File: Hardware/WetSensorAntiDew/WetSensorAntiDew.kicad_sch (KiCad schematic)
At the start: 22 parts, among them J1 Teensy Connector, J2 Connector to BME280, J3 1-4 to HeatedWetSensor | 5-7 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, J4 Teensy Connector, J5 Connector to power supply, J6 Connector to power supply, Q1 MOSFET N-CH, U1 AMS1117

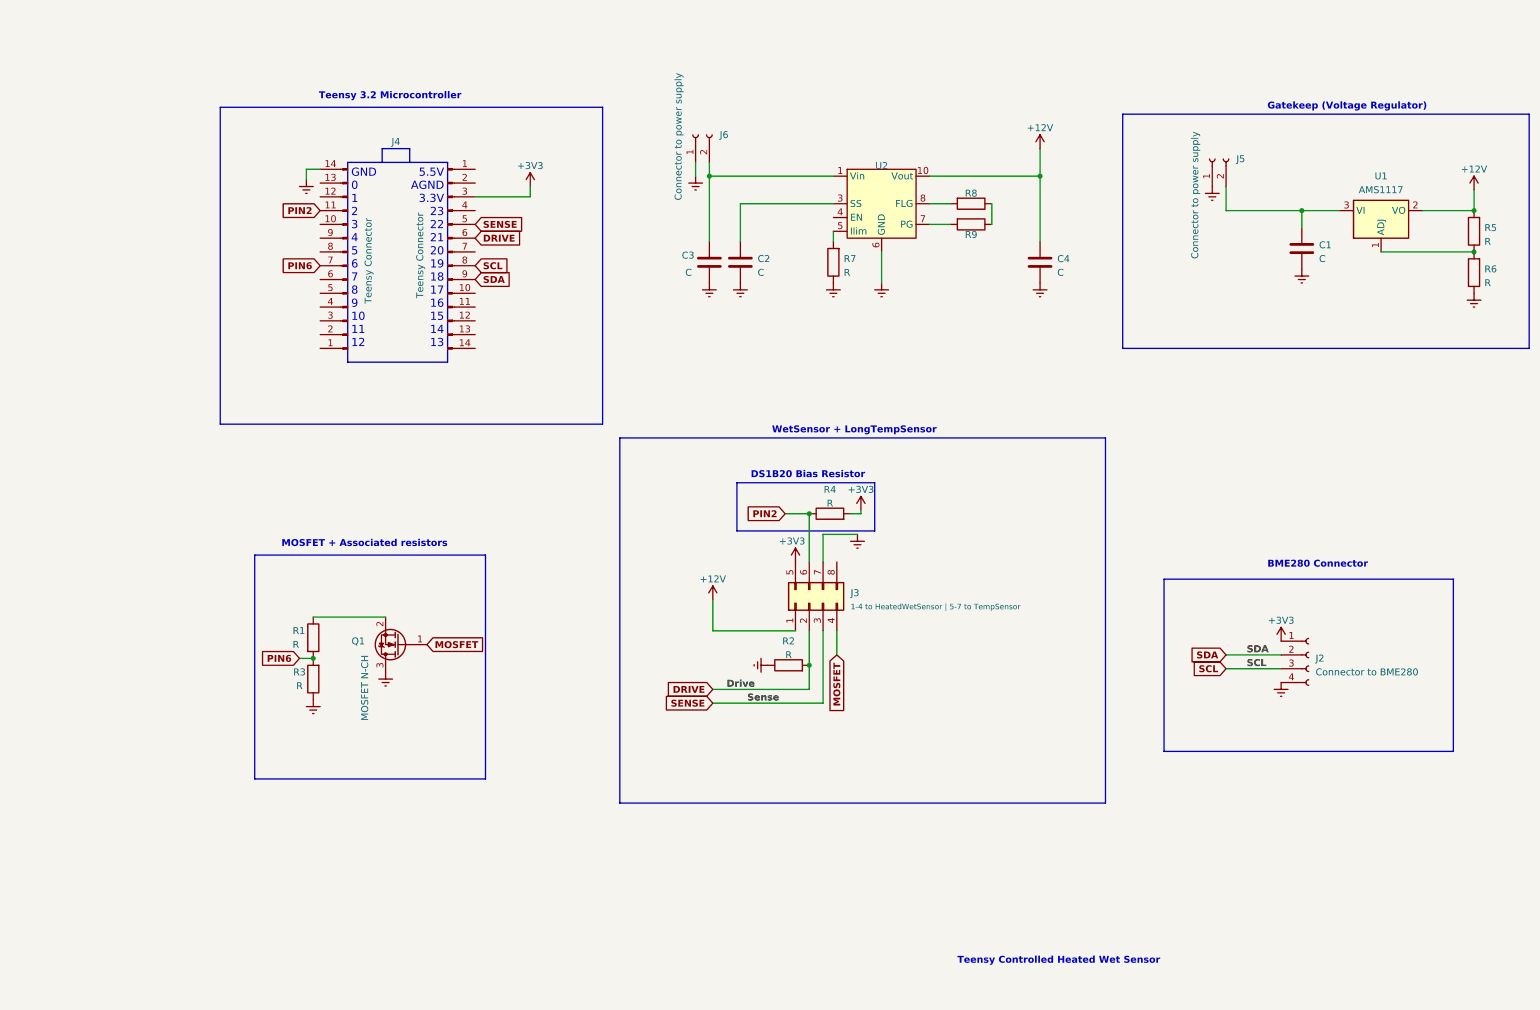
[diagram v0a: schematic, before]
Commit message: changes
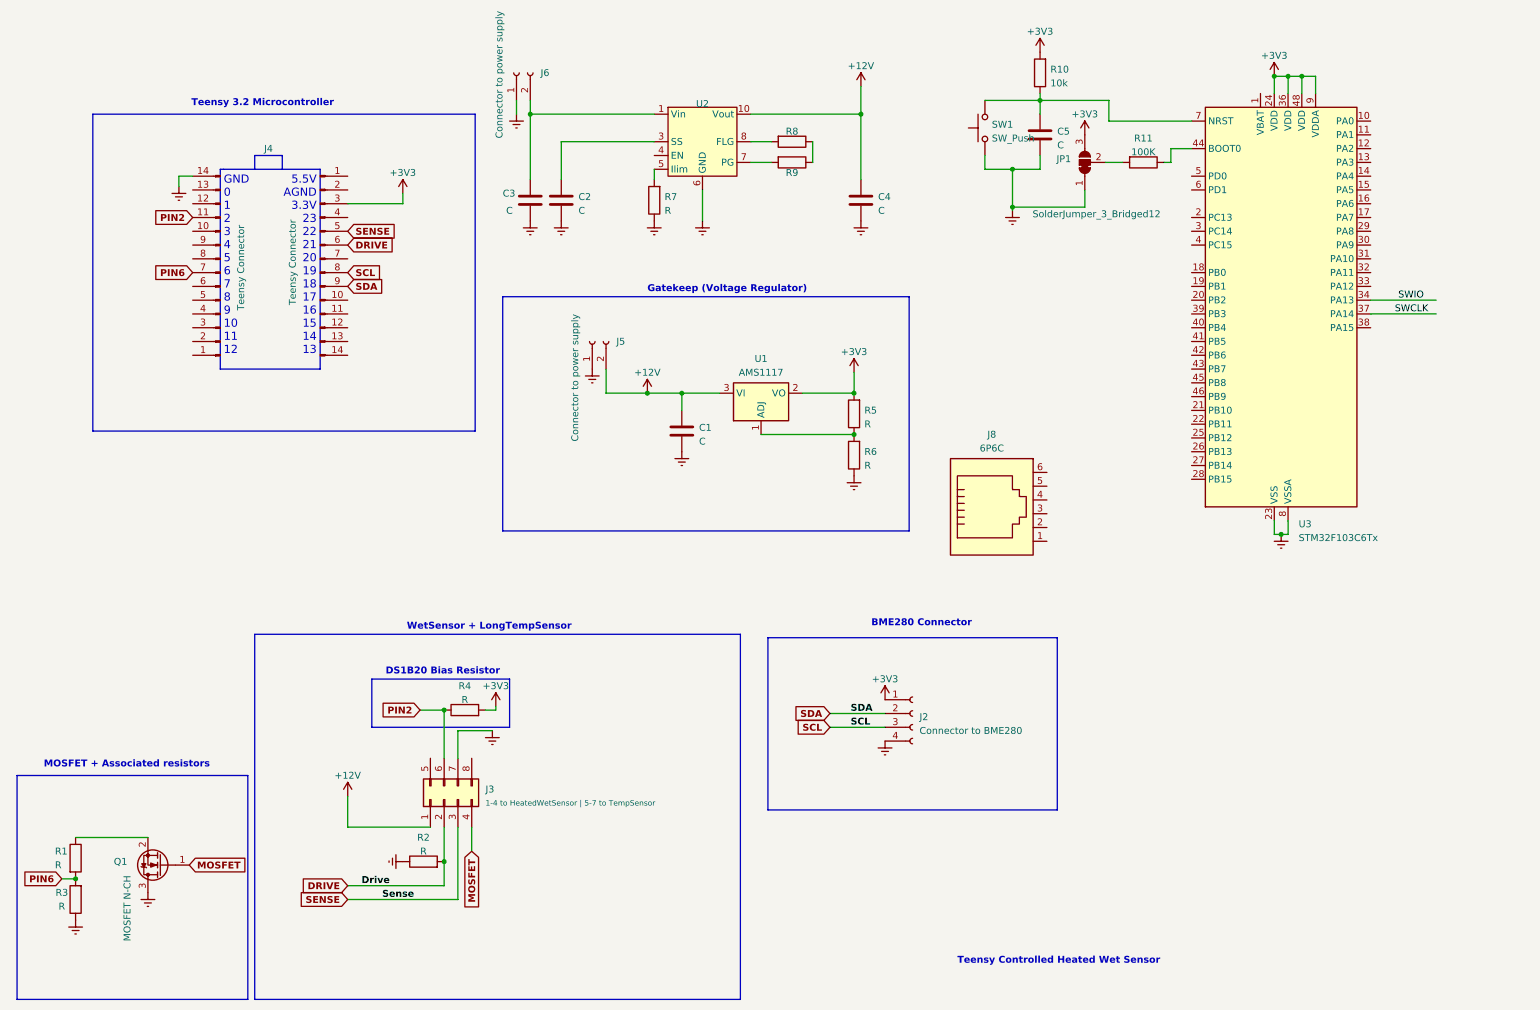
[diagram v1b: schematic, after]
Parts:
- added C5: C, Capacitor_SMD:C_0603_1608Metric_Pad1.08x0.95mm_HandSolder, symbol Device:C
- added J8: 6P6C, Connector_RJ:RJ12_Amphenol_54601, symbol Connector:6P6C
- added JP1: SolderJumper_3_Bridged12, Jumper:SolderJumper-3_P1.3mm_Bridged12_Pad1.0x1.5mm_NumberLabels, symbol Jumper:SolderJumper_3_Bridged12
- added R10: 10k, Resistor_SMD:R_0603_1608Metric_Pad0.98x0.95mm_HandSolder, symbol Device:R
- added R11: 100K, Resistor_SMD:R_0603_1608Metric_Pad0.98x0.95mm_HandSolder, symbol Device:R
- added SW1: SW_Push, symbol Switch:SW_Push
- added U3: STM32F103C6Tx, Package_QFP:LQFP-48_7x7mm_P0.5mm, symbol MCU_ST_STM32F1:STM32F103C6Tx
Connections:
- net +12V: now also C1.1, J5.2 (Pin_2), U1.3 (VI); no longer R5.2, U1.2 (VO)
- net +3V3: now also R5.2, U1.2 (VO), JP1.3 (B), R10.2, U3.24 (VDD), U3.36 (VDD), U3.48 (VDD), U3.9 (VDDA); no longer J3.5 (Pin_5)
- net Earth: now also C5.2, JP1.1 (A), SW1.1, U3.23 (VSS), U3.35 (VSS), U3.47 (VSS), U3.8 (VSSA)
- new net: R11.1, U3.44 (BOOT0)
- new net: C5.1, R10.1, SW1.2, U3.7 (NRST)
- new net: JP1.2 (C), R11.2
- new net SWCLK: U3.37 (PA14)
- new net SWIO: U3.34 (PA13)
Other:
- moved on the sheet: C1, C2, C3, C4, J2, J3, J4, J5, J6, Q1, R1, R2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
